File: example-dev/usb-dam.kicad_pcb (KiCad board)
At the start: 2 copper layers, 44 parts, among them J1 USB_C_Receptacle, J2 Conn_01x08_Pin, U1 MCP6002-xMC, U2 SiP32431DR3, U3 TMUX1574RSVR, U4 74LVC1G08

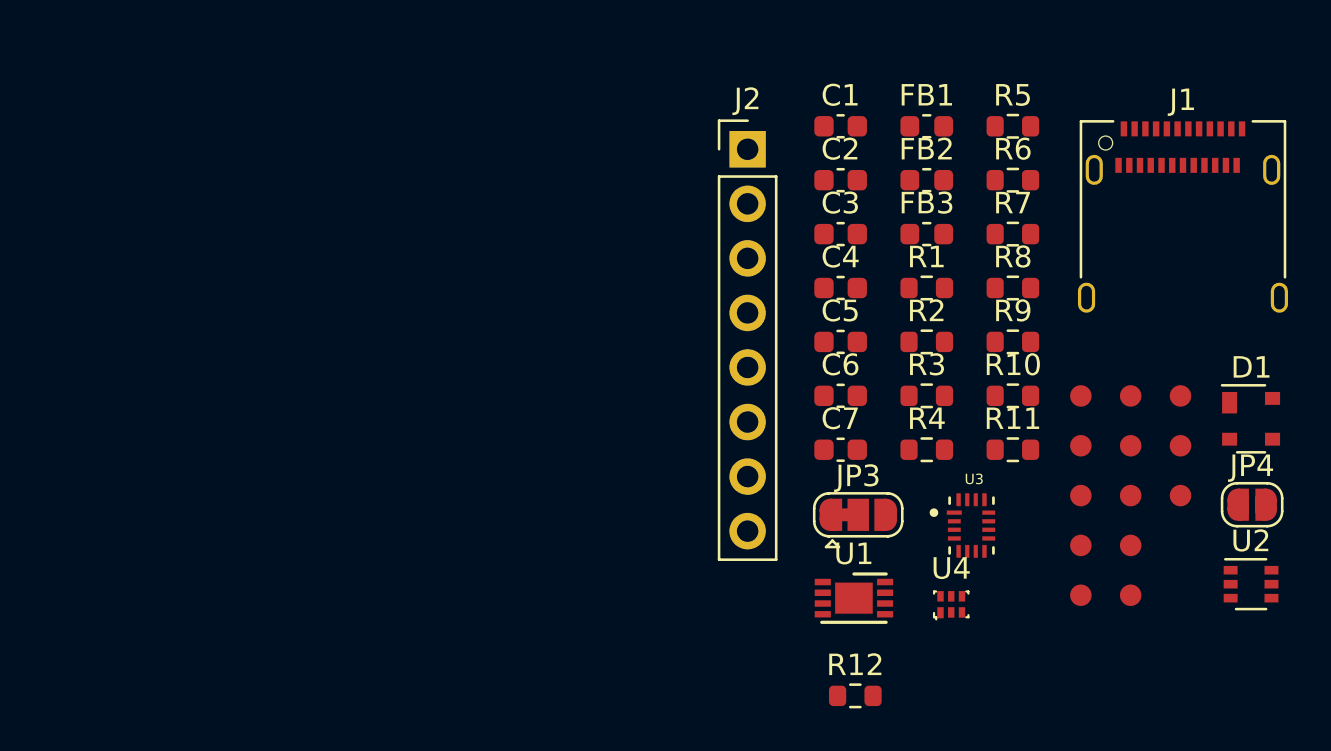
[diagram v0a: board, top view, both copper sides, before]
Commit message: layout example board
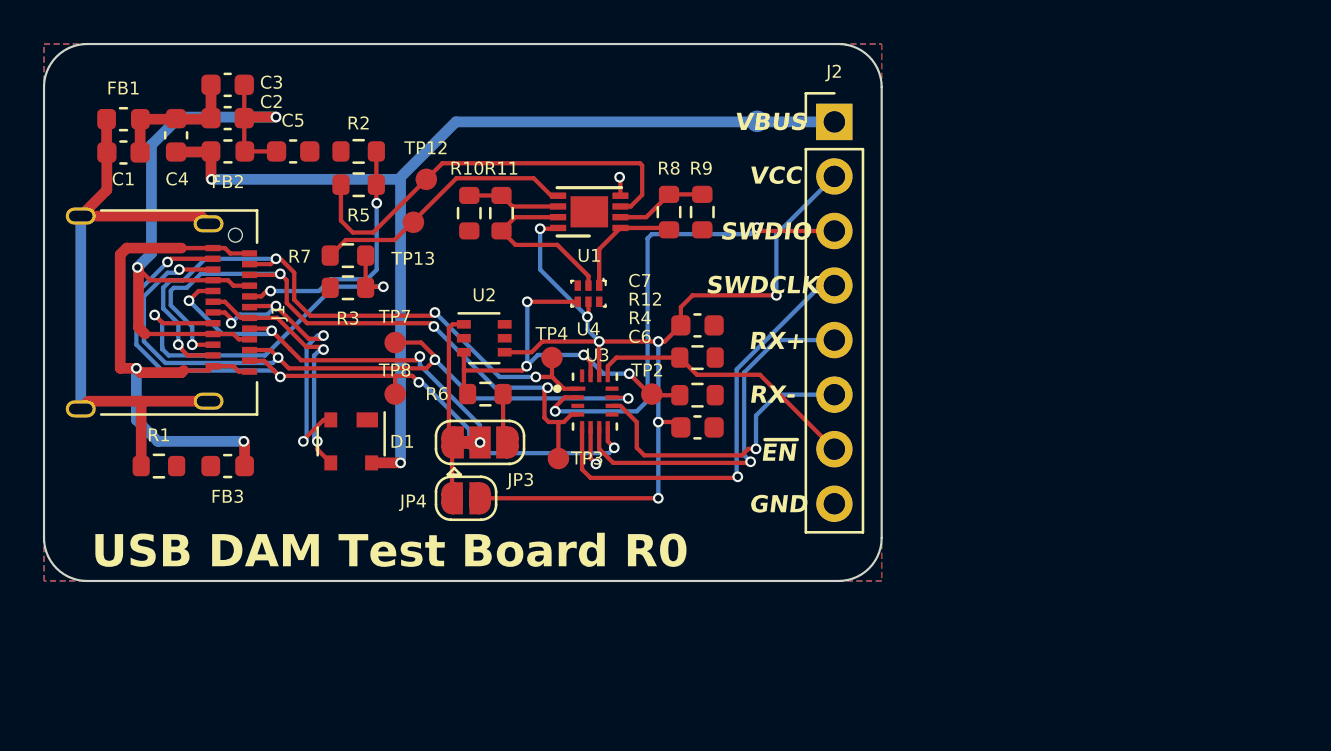
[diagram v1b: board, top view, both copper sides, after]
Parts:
- removed TP1, TP10, TP11, TP6, TP9: TestPoint, tuna-f1sh/jbr-kicad/Misc.pretty:TestPoint_Pad_D1.0mm_Tight
- added G***: LOGO, tuna-f1sh/jbr-kicad/Logos.pretty:jbr-binary-xs-mask, F.Cu at (131.4, 80.7)
- TP5: moved to B.Cu
- moved J1 48.6 mm to (110.5, 90.5), turned to -90 degrees
- moved D1 41.9 mm to (120.3, 96.5), turned to -90 degrees
- moved TP13 37.9 mm to (123.2, 86.3)
- moved U2 37.5 mm to (126.5, 91.7)
- moved FB1 37.4 mm to (109.7, 81.5)
- moved TP12 37.2 mm to (123.8, 84.3)
- moved R1 36.7 mm to (111.3, 97.7)
- moved JP4 36.6 mm to (125.7, 99.2), turned to 180 degrees
- moved TP7 34.6 mm to (122.3, 91.9)
- moved TP8 34.6 mm to (122.3, 94.3)
- moved FB3 34.3 mm to (114.5, 97.7), turned to 180 degrees
- moved C1 33.4 mm to (109.7, 83.0)
- moved FB2 32.6 mm to (114.6, 83.0), turned to 180 degrees
- moved C4 31.7 mm to (112.2, 82.2), turned to 90 degrees
- moved R7 31.0 mm to (120.2, 87.8), turned to 180 degrees
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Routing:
- net VBUS: track 0.00 -> 47.4 mm, vias 0 -> 2
- net VCC: track 0.00 -> 47.2 mm, vias 0 -> 7
- net /RX+: track 0.00 -> 35.3 mm, vias 0 -> 4
- net /RX-: track 0.00 -> 34.5 mm, vias 0 -> 4
- net /VBUS_CONN: track 0.00 -> 32.2 mm, vias 0 -> 2
- net /TX-: track 0.00 -> 31.0 mm, vias 0 -> 4
- net /TX+: track 0.00 -> 30.3 mm, vias 0 -> 4
- net /SHIELD: track 0.00 -> 29.2 mm
- net /USB_GND: track 0.00 -> 26.9 mm, vias 0 -> 2
- net /SWDIO: track 0.00 -> 22.5 mm, vias 0 -> 2
- net /SWDCLK: track 0.00 -> 20.6 mm, vias 0 -> 1
- net /CC1: track 0.00 -> 19.9 mm
- net /DAM_EN: track 0.00 -> 19.6 mm, vias 0 -> 4
- net /SBU: track 0.00 -> 19.6 mm, vias 0 -> 4
- net Net-(J1-CC2): track 0.00 -> 18.8 mm, vias 0 -> 2
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- added copper zone on B.Cu, net GND
- added copper zone on F.Cu, net GND
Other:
- board outline added: 39 x 25 mm
- board text added: "GND"
- board text added: "RX+"
- board text added: "RX-"
- board text added: "SWDCLK"
- board text added: "SWDIO"
- board text added: "USB DAM Test Board R${REVISION}"
- board text added: "VBUS"
- board text added: "VCC"
- board text added: "~{EN}"
